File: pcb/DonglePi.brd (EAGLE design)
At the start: 72.1 x 17.8 mm, 17 parts

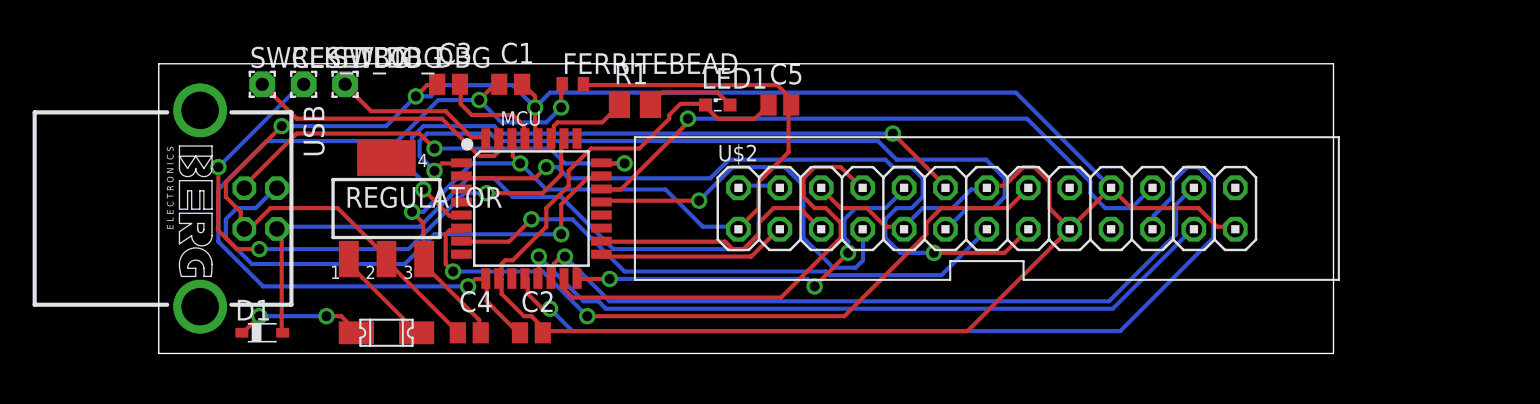
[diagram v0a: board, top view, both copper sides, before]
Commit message: pass on sch
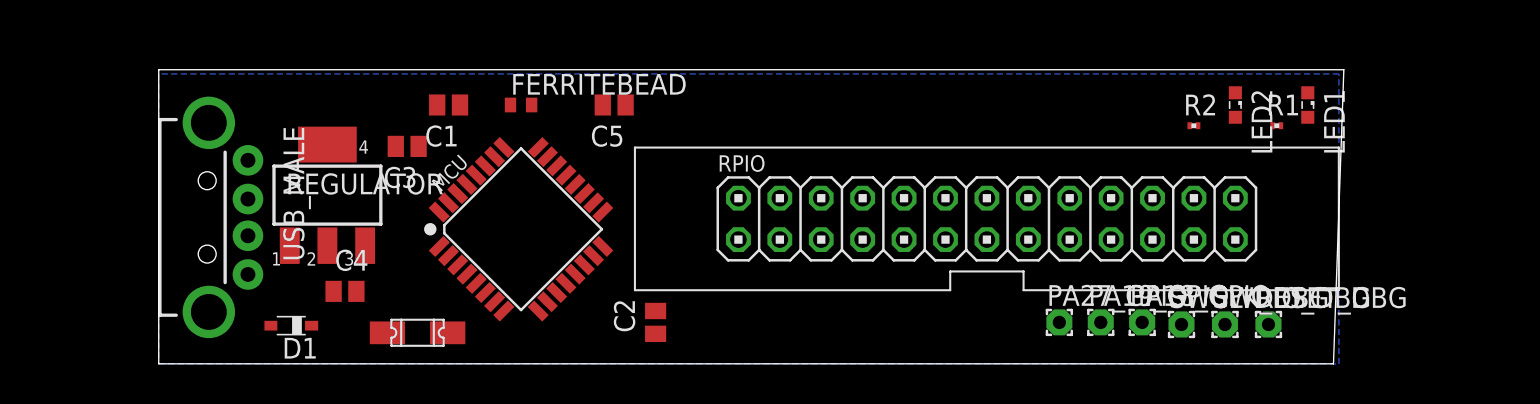
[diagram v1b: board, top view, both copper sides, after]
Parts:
- removed U$2: RPI_2X13, gbin:2X13
- removed USB: PN61729-S, con-berg:PN61729-S
- added LED2: _, eagle-ltspice:LED_SML0603
- added PA18_GPIO, PA19_GPIO, PA27_GPIO: _, wirepad:1,6/0,8
- added R2: 500, eagle-ltspice:R0201
- added RPIO: RPI_2X13, gbin:2X13
- added USB_MALE: USB-A-H, gbin:USB-A-H
- LED1, RESET_DBG, SWCLK_DBG, SWDIO_DBG: value (none) -> _
- R1: device rcl:M0805 -> eagle-ltspice:R0201
- moved RESET_DBG 61.0 mm to (68.1, 1.78)
- moved SWCLK_DBG 58.3 mm to (62.7, 1.78)
- moved SWDIO_DBG 55.9 mm to (65.4, 1.78)
- moved R1 39.4 mm to (68.6, 14.0)
- moved LED1 36.2 mm to (70.5, 15.2), turned to 270 degrees
- moved C5 10.2 mm to (27.9, 15.2), turned to 180 degrees
- moved C4 8.03 mm to (11.4, 3.81)
- moved C2 7.65 mm to (30.5, 1.91), turned to 90 degrees
- moved C3 4.58 mm to (15.2, 12.7), turned to 180 degrees
- moved C1 4.02 mm to (17.8, 15.2), turned to 180 degrees
- moved REGULATOR 3.71 mm to (10.3, 9.71)
- moved FERRITEBEAD 3.42 mm to (22.2, 15.2)
- moved F1 1.90 mm to (15.9, 1.27)
- moved D1 1.83 mm to (8.13, 1.71), turned to 180 degrees
- moved MCU 1.42 mm to (22.2, 7.62), turned to 45 degrees
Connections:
- new net N$6: LED2.A, R2.2
- net +3V3: now also RPIO.1; no longer U$2.1
- net +5V: now also RPIO.2, RPIO.4, USB_MALE.VBUS; no longer U$2.2, U$2.4, USB.1
- net GND: now also LED2.C, RPIO.14, RPIO.17, RPIO.20, RPIO.25, RPIO.6, RPIO.9, USB_MALE.GND; no longer U$2.14, U$2.17, U$2.20, U$2.25, U$2.6, U$2.9, USB.4
- net PA00: now also RPIO.11; no longer U$2.11
- net PA01: now also RPIO.15; no longer U$2.15
- net PA02: now also RPIO.26; no longer U$2.26
- net PA03: now also R2.1
- net PA04: now also RPIO.12; no longer U$2.12
- net PA05: now also RPIO.16; no longer U$2.16
- net PA06: now also RPIO.13; no longer U$2.13
- net PA07: now also RPIO.18; no longer U$2.18
- net PA08: now also RPIO.19; no longer U$2.19
- net PA09: now also RPIO.21; no longer U$2.21
- net PA10: now also RPIO.23; no longer U$2.23
- net PA11: now also RPIO.24; no longer U$2.24
- net PA14: now also RPIO.8; no longer U$2.8
- net PA15: now also RPIO.10; no longer U$2.10
- net PA16: now also RPIO.3; no longer U$2.3
- net PA17: now also RPIO.5; no longer U$2.5
- net PA18: now also PA18_GPIO.1
- net PA19: now also PA19_GPIO.1
- net PA22: now also RPIO.7; no longer U$2.7
- net PA23: now also RPIO.22; no longer U$2.22
- net PA24: now also USB_MALE.D-; no longer USB.2
- net PA25: now also USB_MALE.D+; no longer USB.3
- net PA27: now also PA27_GPIO.1
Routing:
- net GND: track 182.0 -> 0.00 mm, vias 3 -> 0
- net PA09: track 56.6 -> 0.00 mm, vias 1 -> 0
- net +3V3: track 56.3 -> 0.00 mm, vias 2 -> 0
- net N$5: track 52.5 -> 0.00 mm, vias 3 -> 0
- net PA00: track 46.9 -> 0.00 mm, vias 1 -> 0
- net PA11: track 45.5 -> 0.00 mm, vias 1 -> 0
- net +5V: track 45.2 -> 0.00 mm
- net PA10: track 44.9 -> 0.00 mm, vias 1 -> 0
- net PA01: track 44.7 -> 0.00 mm, vias 2 -> 0
- net PA05: track 43.7 -> 0.00 mm, vias 2 -> 0
- net PA04: track 41.1 -> 0.00 mm, vias 2 -> 0
- net PA23: track 38.9 -> 0.00 mm, vias 1 -> 0
- net N$7: track 36.9 -> 0.00 mm, vias 3 -> 0
- net PA06: track 35.4 -> 0.00 mm, vias 1 -> 0
- net PA24: track 32.1 -> 0.00 mm, vias 1 -> 0
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- added copper zone on layer 16, net GND
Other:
- board size 72.1 x 17.8 mm -> 72.7 x 18 mm

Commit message: silkscreen / routing POC
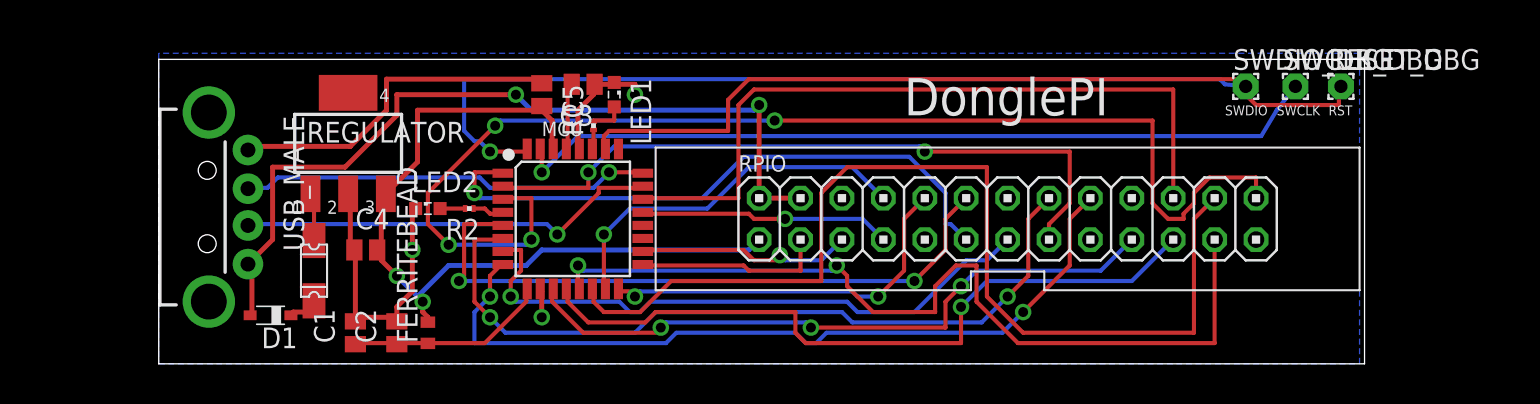
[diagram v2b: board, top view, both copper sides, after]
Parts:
- removed F1: 1206L, gbin:1206L
- removed PA18_GPIO, PA19_GPIO, PA27_GPIO: _, wirepad:1,6/0,8
- added FUSE: 1206L, gbin:1206L
- moved LED2 49.9 mm to (16.5, 8.89), turned to 0 degrees
- moved R2 44.7 mm to (19.1, 8.89), turned to 180 degrees
- moved LED1 42.5 mm to (27.9, 15.9)
- moved R1 41.9 mm to (26.7, 14.0), turned to 90 degrees
- moved SWCLK_DBG 16.2 mm to (69.7, 16.4)
- moved C2 15.9 mm to (14.6, 1.27)
- moved RESET_DBG 15.3 mm to (72.5, 16.4)
- moved C1 15.1 mm to (12.1, 1.27), turned to 90 degrees
- moved FERRITEBEAD 15.1 mm to (16.5, 1.27), turned to 90 degrees
- moved SWDIO_DBG 14.7 mm to (66.7, 16.4)
- moved C3 11.4 mm to (26.0, 16.5)
- moved C5 4.49 mm to (23.5, 15.9), turned to 270 degrees
- moved REGULATOR 3.42 mm to (11.6, 12.9)
- moved MCU 3.24 mm to (25.4, 8.26), turned to 0 degrees
- moved C4 2.84 mm to (12.7, 6.35)
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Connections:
- net N$1: now also FUSE.P$2; no longer F1.P$2
- net N$2: now also FUSE.P$1; no longer F1.P$1
- net PA18: no longer PA18_GPIO.1
- net PA19: no longer PA19_GPIO.1
- net PA27: no longer PA27_GPIO.1
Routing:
- net PA02: track 0.00 -> 74.2 mm, vias 0 -> 4
- net PA11: track 0.00 -> 62.4 mm
- net PA31: track 0.00 -> 55.8 mm, vias 0 -> 1
- net PA10: track 0.00 -> 54.1 mm, vias 0 -> 2
- net +5V: track 0.00 -> 51.1 mm, vias 0 -> 2
- net N$7: track 0.00 -> 50.9 mm
- net PA30: track 0.00 -> 50.2 mm, vias 0 -> 1
- net PA07: track 0.00 -> 49.2 mm, vias 0 -> 2
- net GND: track 0.00 -> 48.8 mm, vias 0 -> 3
- net +3V3: track 0.00 -> 48.3 mm, vias 0 -> 2
- net PA05: track 0.00 -> 47.6 mm, vias 0 -> 2
- net PA23: track 0.00 -> 45.3 mm
- net PA09: track 0.00 -> 44.2 mm, vias 0 -> 1
- net PA01: track 0.00 -> 42.5 mm, vias 0 -> 2
- net PA08: track 0.00 -> 40.9 mm, vias 0 -> 3
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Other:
- board size 72.7 x 18 mm -> 74 x 18.7 mm
- board text added: "DonglePI"
- board text added: "RST"
- board text added: "SWCLK"
- board text added: "SWDIO"
